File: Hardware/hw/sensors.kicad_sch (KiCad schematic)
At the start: 53 parts, among them J11 Screw_Terminal_01x03, J3 Screw_Terminal_01x04, J5 Screw_Terminal_01x04, J6 Screw_Terminal_01x04, J8 Screw_Terminal_01x04, J9 Screw_Terminal_01x04, Q10 NMOS, Q11 NMOS, Q12 NMOS, Q13 NMOS, Q14 NMOS, Q15 NMOS, Q16 NMOS, Q17 NMOS, Q8 NMOS, Q9 NMOS, U10 PESD5V0L2BT,215, U11 PESD5V0L2BT,215, U12 PESD5V0L2BT,215, U3 PESD5V0L2BT,215, U8 PESD5V0L2BT,215

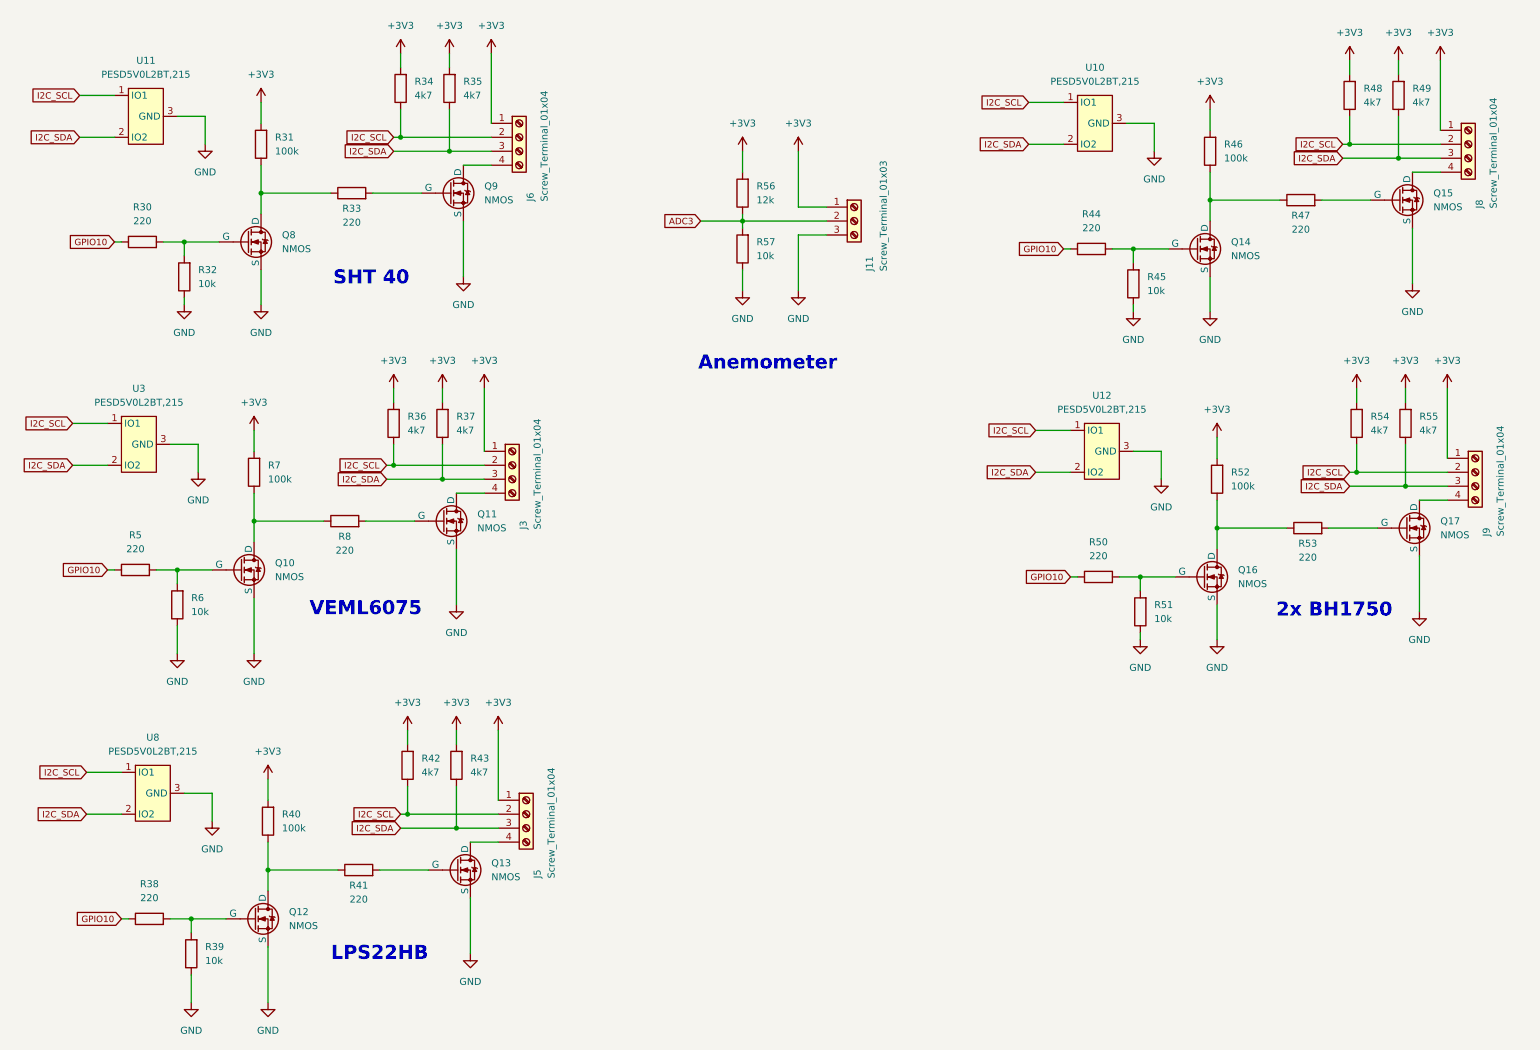
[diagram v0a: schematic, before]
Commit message: Anemometer update
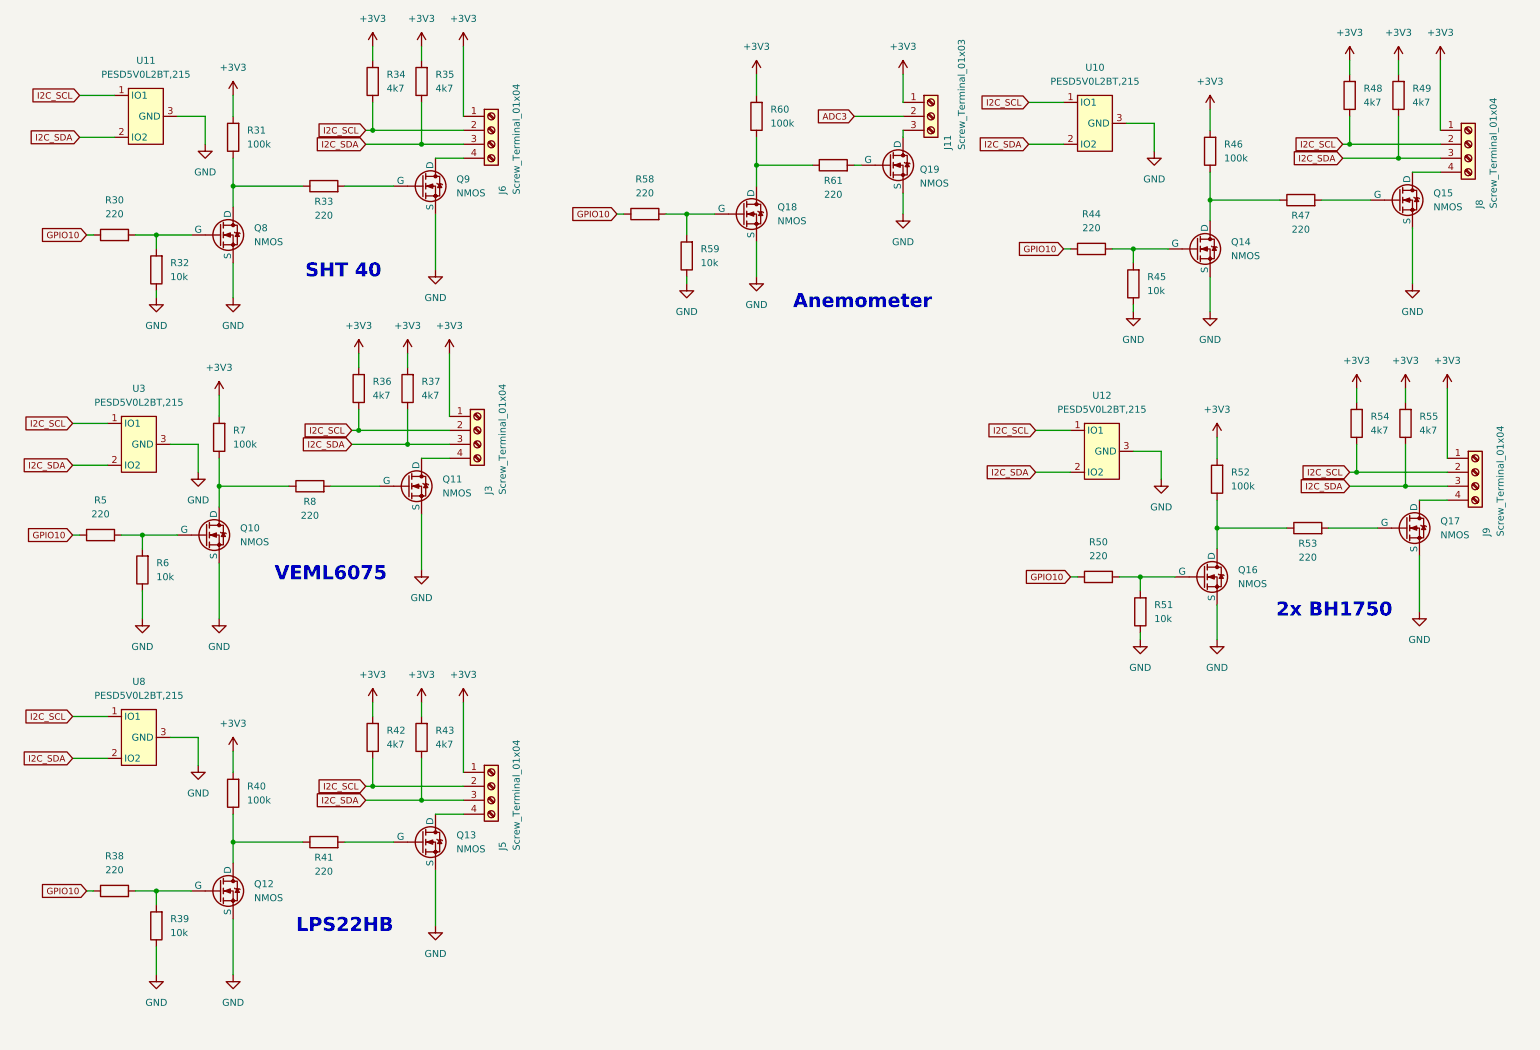
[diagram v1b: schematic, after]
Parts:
- removed R56: 12k, Resistor_SMD:R_0805_2012Metric, symbol Device:R
- removed R57: 10k, Resistor_SMD:R_0805_2012Metric, symbol Device:R
- added Q18, Q19: NMOS, symbol Simulation_SPICE:NMOS
- added R58, R61: 220, Resistor_SMD:R_0805_2012Metric, symbol Device:R
- added R59: 10k, Resistor_SMD:R_0805_2012Metric, symbol Device:R
- added R60: 100k, Resistor_SMD:R_0805_2012Metric, symbol Device:R
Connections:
- net +3V3: now also R60.2
- net GND: now also Q18.3 (S), Q19.3 (S), R59.1; no longer J11.3 (Pin_3)
- net GPIO10: now also R58.1
- new net: J11.3 (Pin_3), Q19.1 (D)
- new net: Q19.2 (G), R61.2
- new net: Q18.1 (D), R60.1, R61.1
- new net: Q18.2 (G), R58.2, R59.2
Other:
- moved on the sheet: J11, J3, J5, J6, Q10, Q11, Q12, Q13, Q8, Q9, R30, R31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

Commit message: Hardware v1.0
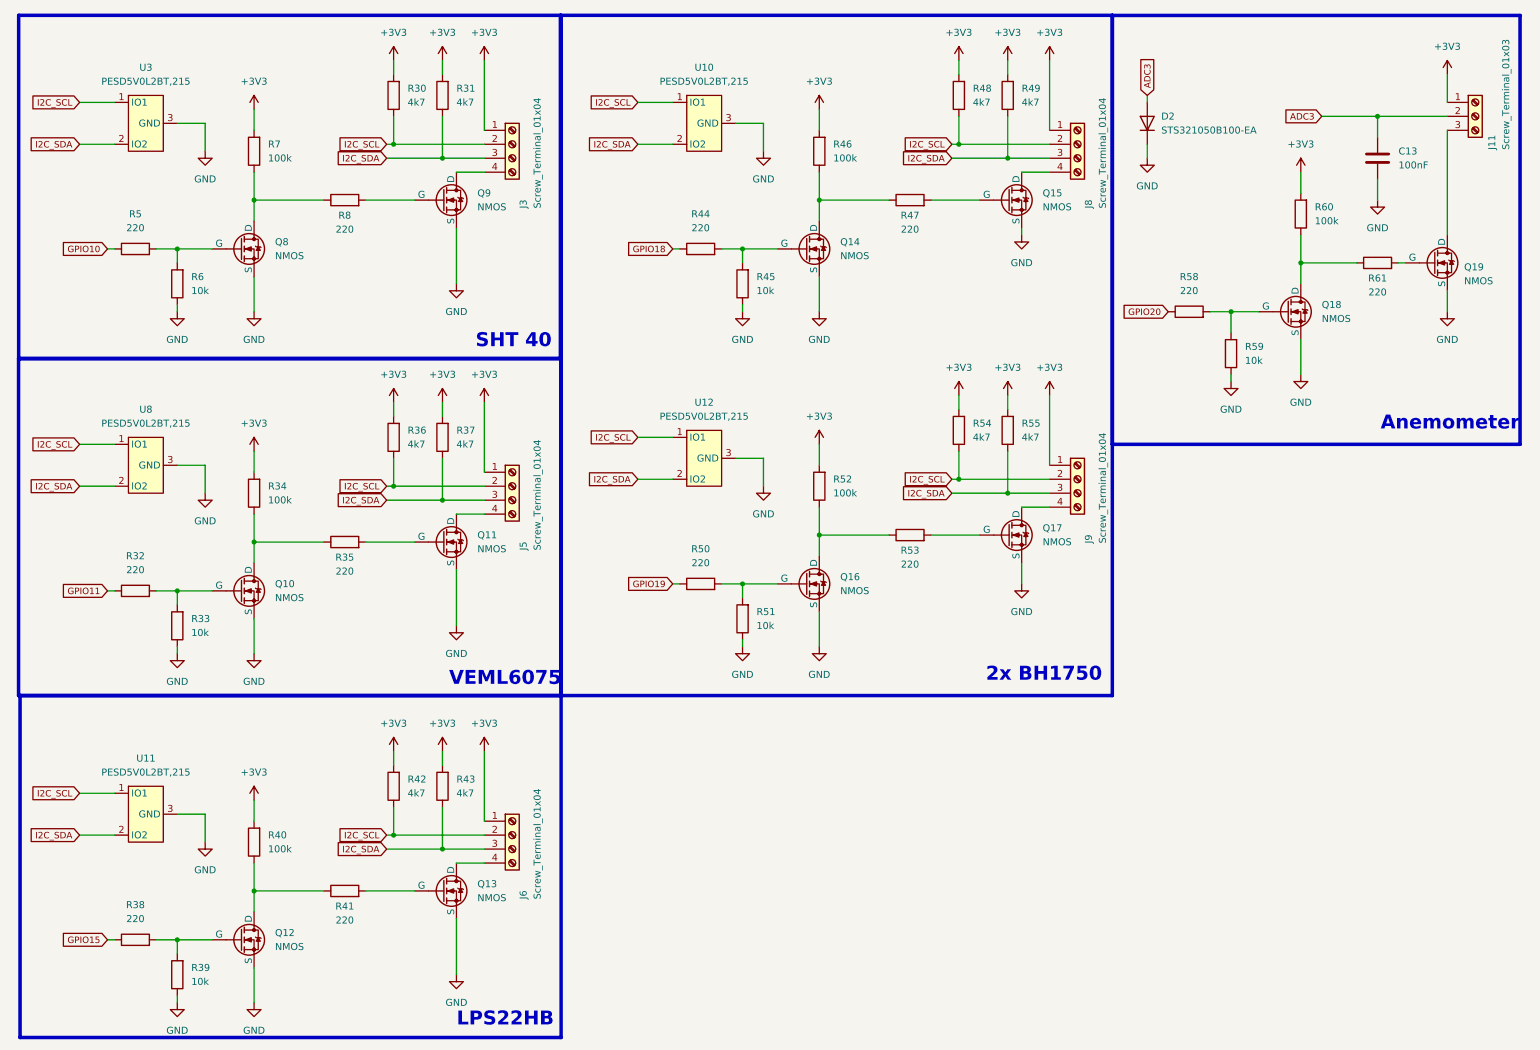
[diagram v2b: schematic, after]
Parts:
- added C13: 100nF, Capacitor_SMD:C_0805_2012Metric, symbol Device:C
- added D2: STS321050B100-EA, Diode_SMD:D_SOD-323, symbol Diode:1N4148WS
- R30: value 220 -> 4k7
- R31: value 100k -> 4k7
- R32: value 10k -> 220
- R33: value 220 -> 10k
- R34: value 4k7 -> 100k
- R35: value 4k7 -> 220
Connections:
- net +3V3: now also R30.2; no longer R35.2
- net ADC3: now also C13.1, D2.2 (A)
- net GND: now also R33.1, C13.2, D2.1 (K); no longer R32.1
- net GPIO10: no longer R30.1, R38.1, R44.1, R50.1, R58.1
- net I2C_SCL: now also R30.1; no longer R34.1
- net I2C_SDA: now also R31.1; no longer R35.1
- net at R7.1, R8.1: now also Q8.1 (D); no longer Q10.1 (D)
- net at Q11.2 (G): now also R35.2; no longer R8.2
- net at R5.2, R6.2: now also Q8.2 (G); no longer Q10.2 (G)
- net at Q9.2 (G): now also R8.2; no longer R33.2
- net at J6.4 (Pin_4): now also Q13.1 (D); no longer Q9.1 (D)
- net at J5.4 (Pin_4): now also Q11.1 (D); no longer Q13.1 (D)
- net at J3.4 (Pin_4): now also Q9.1 (D); no longer Q11.1 (D)
- new net: Q10.1 (D), R34.1, R35.1
- new net: Q10.2 (G), R32.2, R33.2
- new net GPIO11: R32.1
- new net GPIO15: R38.1
- new net GPIO18: R44.1
- new net GPIO19: R50.1
- new net GPIO20: R58.1
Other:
- company: (none) -> UNIZA Faculty of Management Science and Informatics Department of Technical Cybernetics
- title: (none) -> Solar Power Management and Monitoring Circuit
- moved on the sheet: J11, J8, J9, Q14, Q15, Q16, Q17, Q18, Q19, R44, R45, R46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
